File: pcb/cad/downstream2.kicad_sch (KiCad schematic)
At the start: 14 parts, among them J701 USB_C_Receptacle, U701 ECMF02-2AMX6, U702 ECMF02-2AMX6, U703 ECMF02-2AMX6, U704 ECMF02-2AMX6, U705 ECMF02-2AMX6, U706 ECMF02-2AMX6, U707 CBTL02043A, U708 TUSB320, U709 PI3USB221E, U710 LM73100, U711 TPS25947xx

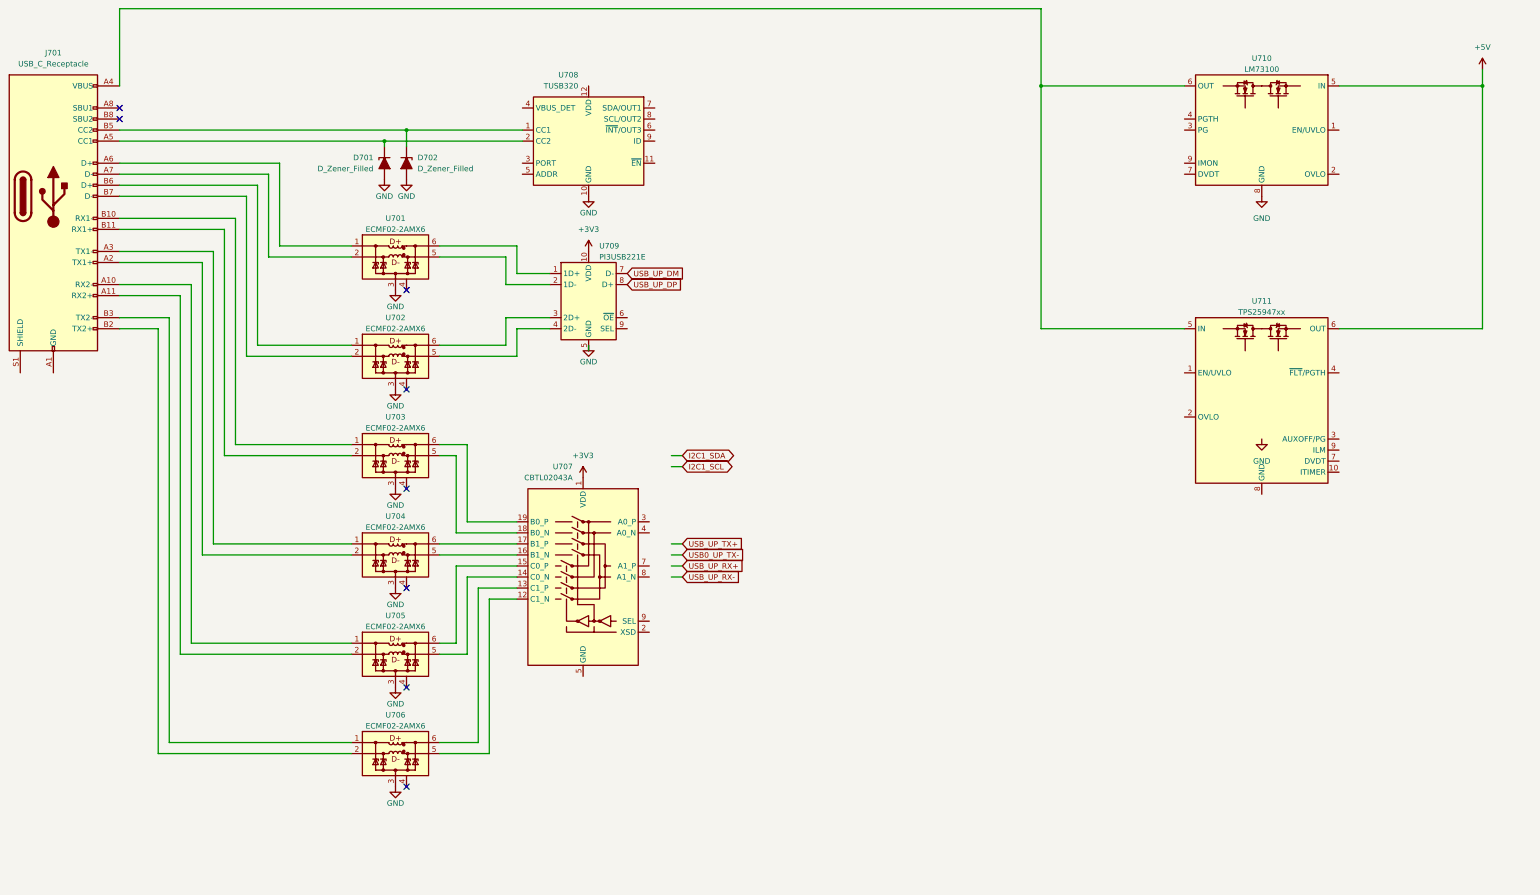
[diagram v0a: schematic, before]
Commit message: moved old-old-old backups and finished preliminary USB architecture
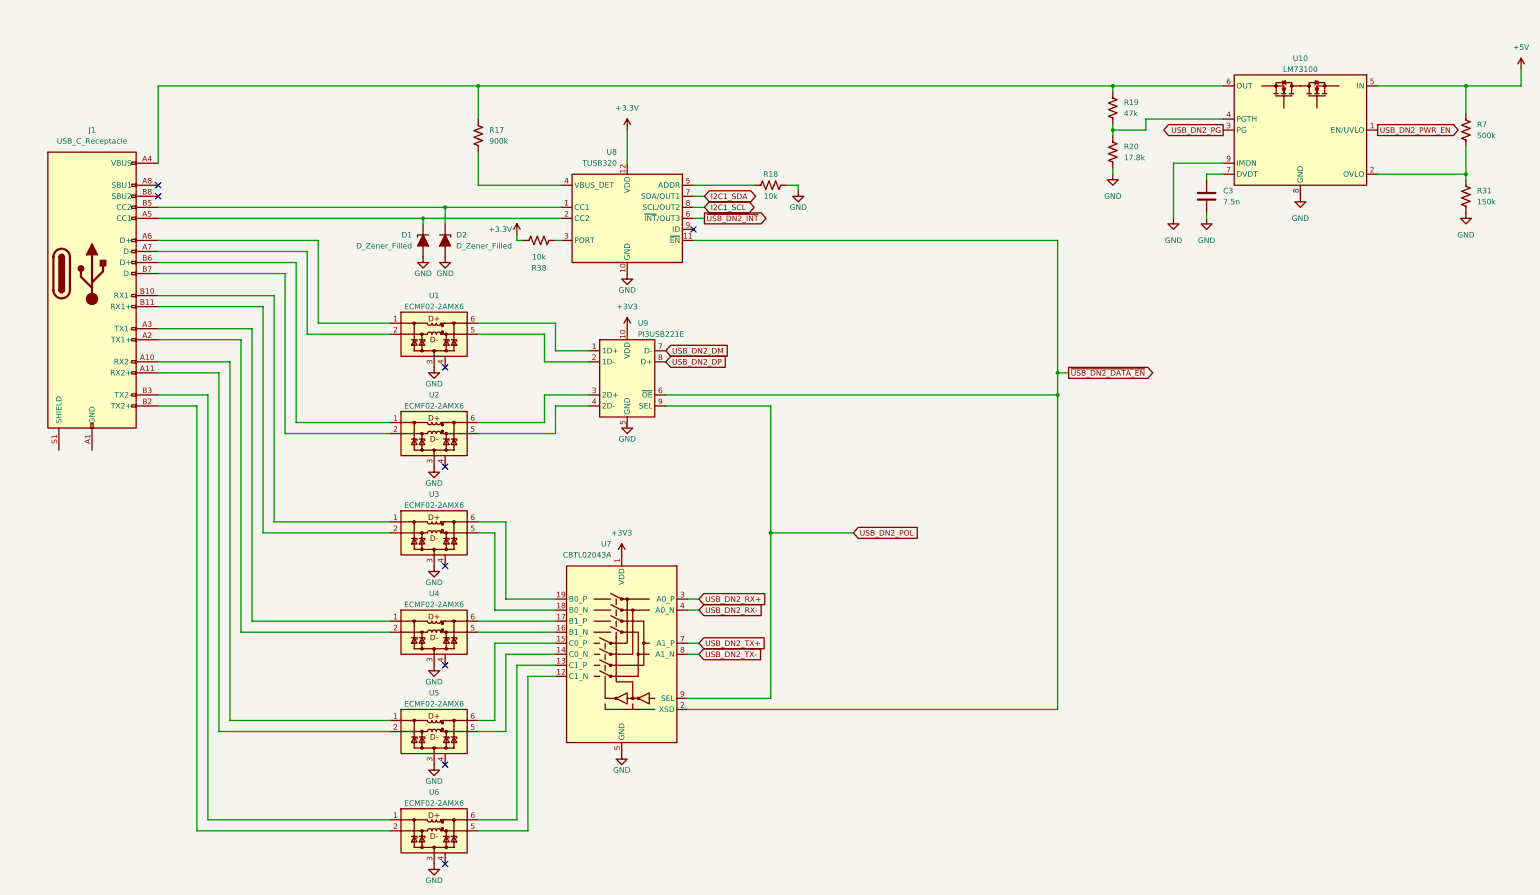
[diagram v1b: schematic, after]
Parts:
- removed D701, D702: D_Zener_Filled, symbol Device:D_Zener_Filled
- removed J701: USB_C_Receptacle, symbol Connector:USB_C_Receptacle
- removed U701, U702, U703, U704, U705, U706: ECMF02-2AMX6, Package_DFN_QFN:ST_UQFN-6L_1.5x1.7mm_P0.5mm, symbol Power_Protection:ECMF02-2AMX6
- removed U707: CBTL02043A, Package_DFN_QFN:WQFN-20-1EP_2.5x4.5mm_P0.5mm_EP1x2.9mm, symbol Analog_Switch:CBTL02043A
- removed U708: TUSB320, Package_DFN_QFN:Texas_X2QFN-12_1.6x1.6mm_P0.4mm, symbol Interface_USB:TUSB320
- removed U709: PI3USB221E, symbol Library:DIODES_PI3USB221E
- removed U710: LM73100, symbol Library:TI_LM73100
- removed U711: TPS25947xx, symbol Library:TI_TPS25947
- added C3: 7.5n, symbol Device:C
- added D1, D2: D_Zener_Filled, symbol Device:D_Zener_Filled
- added J1: USB_C_Receptacle, symbol Connector:USB_C_Receptacle
- added R17: 900k, symbol Device:R_US
- added R18, R38: 10k, symbol Device:R_US
- added R19: 47k, symbol Device:R_US
- added R20: 17.8k, symbol Device:R_US
- added R31: 150k, symbol Device:R_US
- added R7: 500k, symbol Device:R_US
- added U1, U2, U3, U4, U5, U6: ECMF02-2AMX6, Package_DFN_QFN:ST_UQFN-6L_1.5x1.7mm_P0.5mm, symbol Power_Protection:ECMF02-2AMX6
- added U10: LM73100, symbol Library:TI_LM73100
- added U7: CBTL02043A, Package_DFN_QFN:WQFN-20-1EP_2.5x4.5mm_P0.5mm_EP1x2.9mm, symbol Analog_Switch:CBTL02043A
- added U8: TUSB320, Package_DFN_QFN:Texas_X2QFN-12_1.6x1.6mm_P0.4mm, symbol Interface_USB:TUSB320
- added U9: PI3USB221E, symbol Library:DIODES_PI3USB221E
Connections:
- net +3V3: now also U7.1 (VDD), U7.10 (VDD), U7.6 (VDD), U9.10 (VDD)
- net +5V: now also R7.1, U10.5 (IN)
- net GND: now also C3.2, D1.2 (A), D2.2 (A), R18.1, R20.2, R31.2, U1.3 (GND), U10.8 (GND), U10.9 (IMON), U2.3 (GND), U3.3 (GND), U4.3 (GND), U5.3 (GND), U6.3 (GND), U7.11 (GND), U7.20 (GND), U7.21 (GND), U7.5 (GND), U8.10 (GND), U9.5 (GND)
- net I2C1_SCL: now also U8.8 (SCL/OUT2)
- net I2C1_SDA: now also U8.7 (SDA/OUT1)
- new net: U6.5 (D-_out), U7.12 (C1_N)
- new net: U6.6 (D+_out), U7.13 (C1_P)
- new net: U5.5 (D-_out), U7.14 (C0_N)
- new net: U5.6 (D+_out), U7.15 (C0_P)
- new net: U4.5 (D-_out), U7.16 (B1_N)
- new net: U4.6 (D+_out), U7.17 (B1_P)
- new net: U3.5 (D-_out), U7.18 (B0_N)
- new net: U3.6 (D+_out), U7.19 (B0_P)
- new net: R38.1, U8.3 (PORT)
- new net: J1.B6 (D+), U2.1 (D+_in)
- new net: J1.B7 (D-), U2.2 (D-_in)
- new net: U2.5 (D-_out), U9.4 (2D-)
- new net: U2.6 (D+_out), U9.3 (2D+)
- new net: R18.2, U8.5 (ADDR)
- new net: D2.1 (K), J1.B5 (CC2), U8.1 (CC1)
- new net: D1.1 (K), J1.A5 (CC1), U8.2 (CC2)
- new net: R17.2, U8.4 (VBUS_DET)
- new net: C3.1, U10.7 (DVDT)
- new net: J1.A4 (VBUS), J1.A9 (VBUS), J1.B4 (VBUS), J1.B9 (VBUS), R17.1, R19.1, U10.6 (OUT)
- new net: J1.A6 (D+), U1.1 (D+_in)
- new net: J1.A7 (D-), U1.2 (D-_in)
- new net: U1.5 (D-_out), U9.2 (1D-)
- new net: U1.6 (D+_out), U9.1 (1D+)
- new net: R19.2, R20.1, U10.4 (PGTH)
- new net: J1.B3 (TX2-), U6.1 (D+_in)
- new net: J1.B2 (TX2+), U6.2 (D-_in)
- new net: R31.1, R7.2, U10.2 (OVLO)
- new net: J1.A1 (GND), J1.A12 (GND), J1.B1 (GND), J1.B12 (GND)
- new net: J1.A10 (RX2-), U5.1 (D+_in)
- new net: J1.A11 (RX2+), U5.2 (D-_in)
- new net: J1.A2 (TX1+), U4.2 (D-_in)
- new net: J1.A3 (TX1-), U4.1 (D+_in)
- new net: J1.B10 (RX1-), U3.1 (D+_in)
- new net: J1.B11 (RX1+), U3.2 (D-_in)
- new net +3.3V: R38.2, U8.12 (VDD)
- new net USB_DN2_DM: U9.7 (D-)
- new net USB_DN2_DP: U9.8 (D+)
- new net USB_DN2_PG: U10.3 (PG)
- new net USB_DN2_POL: U7.9 (SEL), U9.9 (SEL)
- new net USB_DN2_PWR_EN: U10.1 (EN/UVLO)
- new net USB_DN2_RX+: U7.3 (A0_P)
- new net USB_DN2_RX-: U7.4 (A0_N)
- new net USB_DN2_TX+: U7.7 (A1_P)
- new net USB_DN2_TX-: U7.8 (A1_N)
- new net ~{USB_DN2_DATA_EN}: U7.2 (XSD), U8.11 (~{EN}), U9.6 (~{OE})
- new net ~{USB_DN2_INT}: U8.6 (~{INT}/OUT3)
- no-connect marks 8 -> 9
